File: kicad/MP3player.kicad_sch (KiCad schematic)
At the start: 0 parts

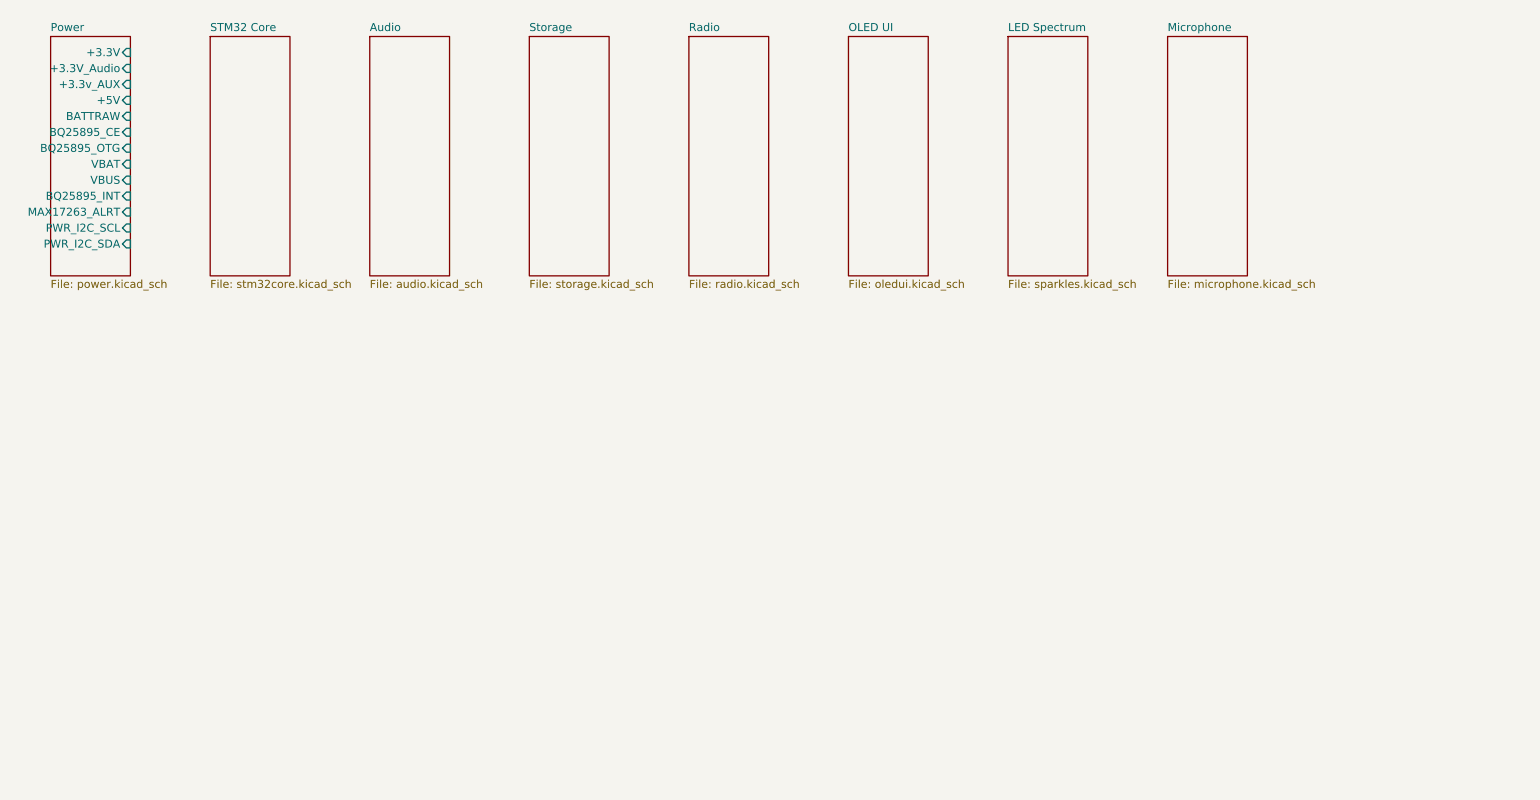
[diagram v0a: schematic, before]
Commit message: changes
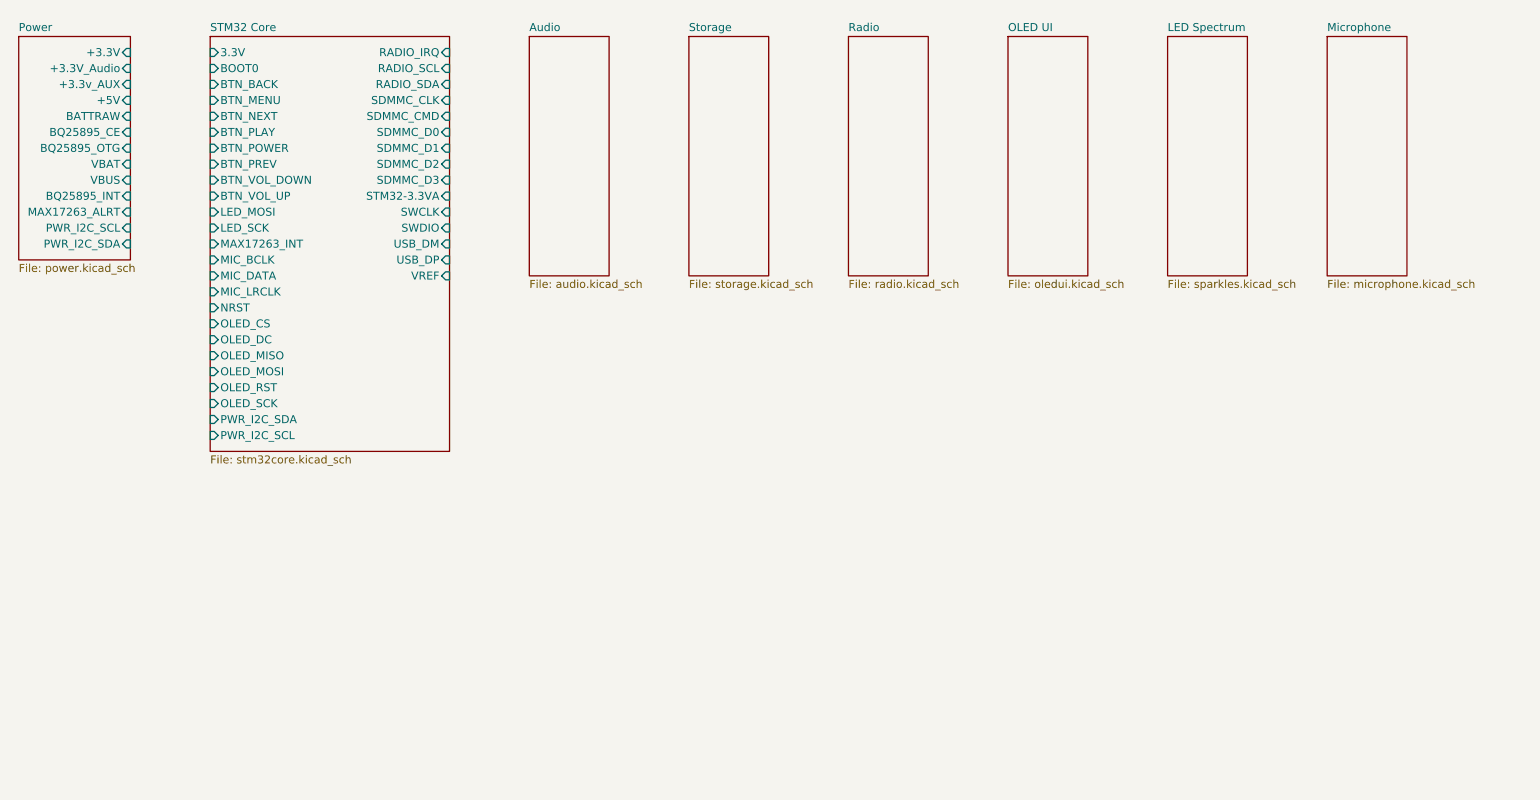
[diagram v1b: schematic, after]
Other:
- sheet STM32 Core ports: added 3.3V, BOOT0, BTN_BACK, BTN_MENU, BTN_NEXT, BTN_PLAY, BTN_POWER, BTN_PREV, BTN_VOL_DOWN, BTN_VOL_UP, LED_MOSI, LED_SCK, MAX17263_INT, MIC_BCLK, MIC_DATA, MIC_LRCLK, NRST, OLED_CS, OLED_DC, OLED_MISO, OLED_MOSI, OLED_RST, OLED_SCK, PWR_I2C_SCL, PWR_I2C_SDA, RADIO_IRQ, RADIO_SCL, RADIO_SDA, SDMMC_CLK, SDMMC_CMD, SDMMC_D0, SDMMC_D1, SDMMC_D2, SDMMC_D3, STM32-3.3VA, SWCLK, SWDIO, USB_DM, USB_DP, VREF; removed none

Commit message: almost done schematic
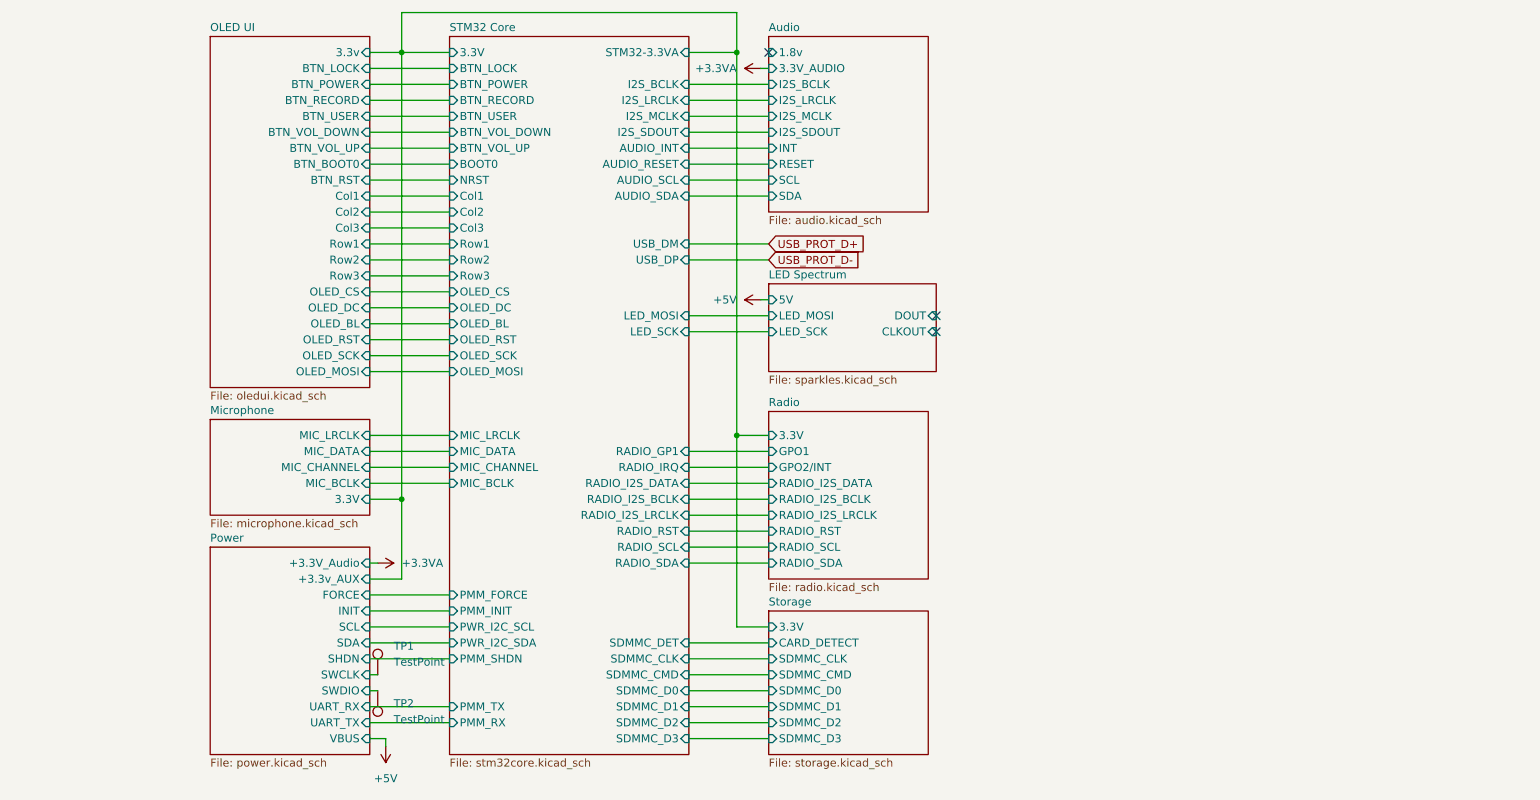
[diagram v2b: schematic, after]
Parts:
- added TP1, TP2: TestPoint, symbol Connector:TestPoint
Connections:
- new net Power/SWCLK: TP1.1
- new net Power/SWDIO: TP2.1
- no-connect marks 0 -> 3
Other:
- sheet Audio ports: added 1.8v, 3.3V_AUDIO, I2S_BCLK, I2S_LRCLK, I2S_MCLK, I2S_SDOUT, INT, RESET, SCL, SDA; removed none
- sheet LED Spectrum ports: added 5V, CLKOUT, DOUT, LED_MOSI, LED_SCK; removed none
- sheet Microphone ports: added 3.3V, MIC_BCLK, MIC_CHANNEL, MIC_DATA, MIC_LRCLK; removed none
- sheet OLED UI ports: added 3.3v, BTN_BOOT0, BTN_LOCK, BTN_POWER, BTN_RECORD, BTN_RST, BTN_USER, BTN_VOL_DOWN, BTN_VOL_UP, Col1, Col2, Col3, OLED_BL, OLED_CS, OLED_DC, OLED_MOSI, OLED_RST, OLED_SCK, Row1, Row2, Row3; removed none
- sheet Power ports: added FORCE, INIT, SCL, SDA, SHDN, SWCLK, SWDIO, UART_RX, UART_TX; removed +3.3V, +5V, BATTRAW, BQ25895_CE, BQ25895_INT, BQ25895_OTG, MAX17263_ALRT, PWR_I2C_SCL, PWR_I2C_SDA, VBAT
- sheet Radio ports: added 3.3V, GPO1, GPO2/INT, RADIO_I2S_BCLK, RADIO_I2S_DATA, RADIO_I2S_LRCLK, RADIO_RST, RADIO_SCL, RADIO_SDA; removed none
- sheet STM32 Core ports: added AUDIO_INT, AUDIO_RESET, AUDIO_SCL, AUDIO_SDA, BTN_LOCK, BTN_RECORD, BTN_USER, Col1, Col2, Col3, I2S_BCLK, I2S_LRCLK, I2S_MCLK, I2S_SDOUT, MIC_CHANNEL, OLED_BL, PMM_FORCE, PMM_INIT, PMM_RX, PMM_SHDN, PMM_TX, RADIO_GP1, RADIO_I2S_BCLK, RADIO_I2S_DATA, RADIO_I2S_LRCLK, RADIO_RST, Row1, Row2, Row3, SDMMC_DET; removed BTN_BACK, BTN_MENU, BTN_NEXT, BTN_PLAY, BTN_PREV, MAX17263_INT, OLED_MISO, SWCLK, SWDIO, VREF
- sheet Storage ports: added 3.3V, CARD_DETECT, SDMMC_CLK, SDMMC_CMD, SDMMC_D0, SDMMC_D1, SDMMC_D2, SDMMC_D3; removed none
